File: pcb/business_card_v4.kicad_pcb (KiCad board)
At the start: 16 copper layers, 89 x 51 mm, 69 parts, among them J1 Conn_01x05_Male, J2 Conn_01x01_Male, SW1 SW_SPST, U1 MIC5504-3.3YM5, U2 STM32G030F6P6

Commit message: create a net and update version of file names
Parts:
- removed JP1: USBPCB, business_card_v1:USB-A-PCB
- added J3: USB_A, Kevin-Lutzer-Kicad-Lbr:USB-A-PCB, F.Cu at (112.0, 122.5)
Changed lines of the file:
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@@
     (add_net SWDIO)
+  )
+  (module Kevin-Lutzer-Kicad-Lbr:USB-A-PCB (layer Top)
+    (at 111.96828 122.5423 45)
+    (descr "Card-edge USB A connector.\n\nFor boards designed to be plugged directly into a USB slot. If possible, ensure that your PCB is about 2.4mm thick to fit snugly.")
+    (fp_text reference J3 (at 0 -7.1 45) (layer F.SilkS) hide
+      (effects (font (size 1.27 1.27) (thickness 0.15)))
+    )
+    (fp_text value USB_A (at 0 7.5 45) (layer F.SilkS) hide
+      (effects (font (size 1.27 1.27) (thickness 0.15)))
+    )
+    (fp_line (start -5 6) (end -5 -6) (layer F.Fab) (width 0.127))
+    (fp_line (start 3.7 6) (end -5 6) (layer F.Fab) (width 0.127))
+    (fp_line (start 3.7 -6) (end 3.7 6) (layer F.Fab) (width 0.127))
+    (fp_line (start -5 -6) (end 3.7 -6) (layer F.Fab) (width 0.127))
+    (pad 4 smd rect (at -0.2 -3.5 45) (size 7.5 1.5) (layers Top F.Paste F.Mask)
+      (net 1 GND) (solder_mask_margin 0.1016))
+    (pad 3 smd rect (at 0.3 -1 45) (size 6.5 1) (layers Top F.Paste F.Mask)
+      (solder_mask_margin 0.1016))
+    (pad 2 smd rect (at 0.3 1 45) (size 6.5 1) (layers Top F.Paste F.Mask)
+      (solder_mask_margin 0.1016))
+    (pad 1 smd rect (at -0.2 3.5 45) (size 7.5 1.5) (layers Top F.Paste F.Mask)
+      (net 2 +5V) (solder_mask_margin 0.1016))
   )
   (module Resistor_SMD:R_0805_2012Metric (layer Top)
@@
     )
   )
-  (module business_card_v1:USB-A-PCB (layer Top)
-    (at 111.96828 122.5423 45)
-    (descr "Card-edge USB A connector.\n\nFor boards designed to be plugged directly into a USB slot. If possible, ensure that your PCB is about 2.4mm thick to fit snugly.")
-    (fp_text reference JP1 (at 0 0 45) (layer F.SilkS) hide
-      (effects (font (size 1.27 1.27) (thickness 0.15)))
-    )
-    (fp_text value USBPCB (at -1.270002 5.079999 45) (layer F.SilkS) hide
-      (effects (font (size 0.38608 0.38608) (thickness 0.030886)))
-    )
-    (fp_text user "Card edge" (at -6.392146 -3.543609 135) (layer Cmts.User) hide
-      (effects (font (size 0.9652 0.9652) (thickness 0.08128)) (justify left bottom))
-    )
-    (fp_text user >Value (at -1.27 5.08 45) (layer F.Fab) hide
-      (effects (font (size 0.38608 0.38608) (thickness 0.032512)) (justify left bottom))
-    )
-    (fp_text user >Name (at -1.27 -5.08 45) (layer F.SilkS) hide
-      (effects (font (size 0.38608 0.38608) (thickness 0.032512)) (justify left bottom))
-    )
-    (fp_line (start -5 6) (end -5 -6) (layer F.Fab) (width 0.127))
-    (fp_line (start 3.7 6) (end -5 6) (layer F.Fab) (width 0.127))
-    (fp_line (start 3.7 -6) (end 3.7 6) (layer F.Fab) (width 0.127))
-    (fp_line (start -5 -6) (end 3.7 -6) (layer F.Fab) (width 0.127))
-    (pad GND smd rect (at -0.2 -3.5 45) (size 7.5 1.5) (layers Top F.Paste F.Mask)
-      (net 1 GND) (solder_mask_margin 0.1016))
-    (pad USB_P smd rect (at 0.3 -1 45) (size 6.5 1) (layers Top F.Paste F.Mask)
-      (solder_mask_margin 0.1016))
-    (pad USB_M smd rect (at 0.3 1 45) (size 6.5 1) (layers Top F.Paste F.Mask)
-      (solder_mask_margin 0.1016))
-    (pad 5V smd rect (at -0.2 3.5 45) (size 7.5 1.5) (layers Top F.Paste F.Mask)
-      (net 2 +5V) (solder_mask_margin 0.1016))
-  )
   (module Button_Switch_SMD:SW_Push_1P1T_NO_CK_KMR2 (layer Top)
     (at 146.2 121.5)
@@
     (effects (font (size 1 1) (thickness 0.14224)))
   )
-  (gr_text 5v-SUP (at 122 110.85) (layer B.SilkS)
+  (gr_text 5v-SUP (at 121.9 110.85) (layer B.SilkS)
     (effects (font (size 1 1) (thickness 0.14224)) (justify mirror))
   )

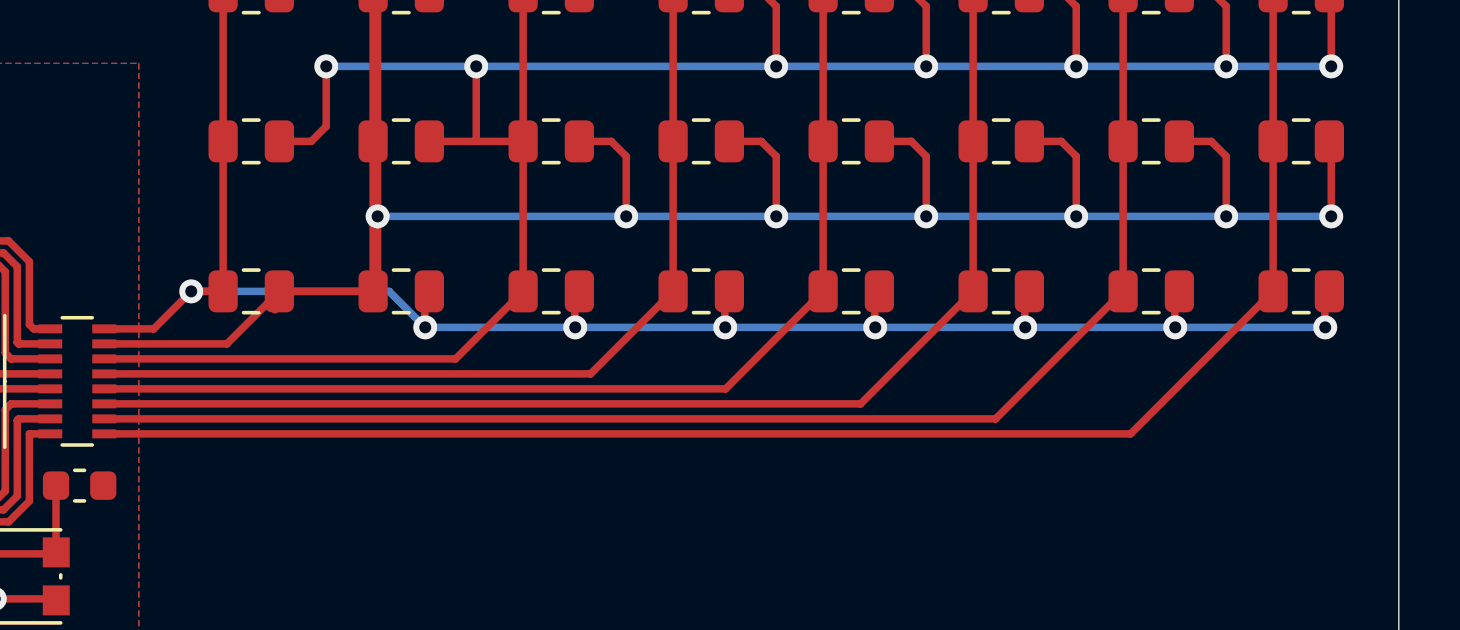
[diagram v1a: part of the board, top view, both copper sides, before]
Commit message: update pcb gerbers
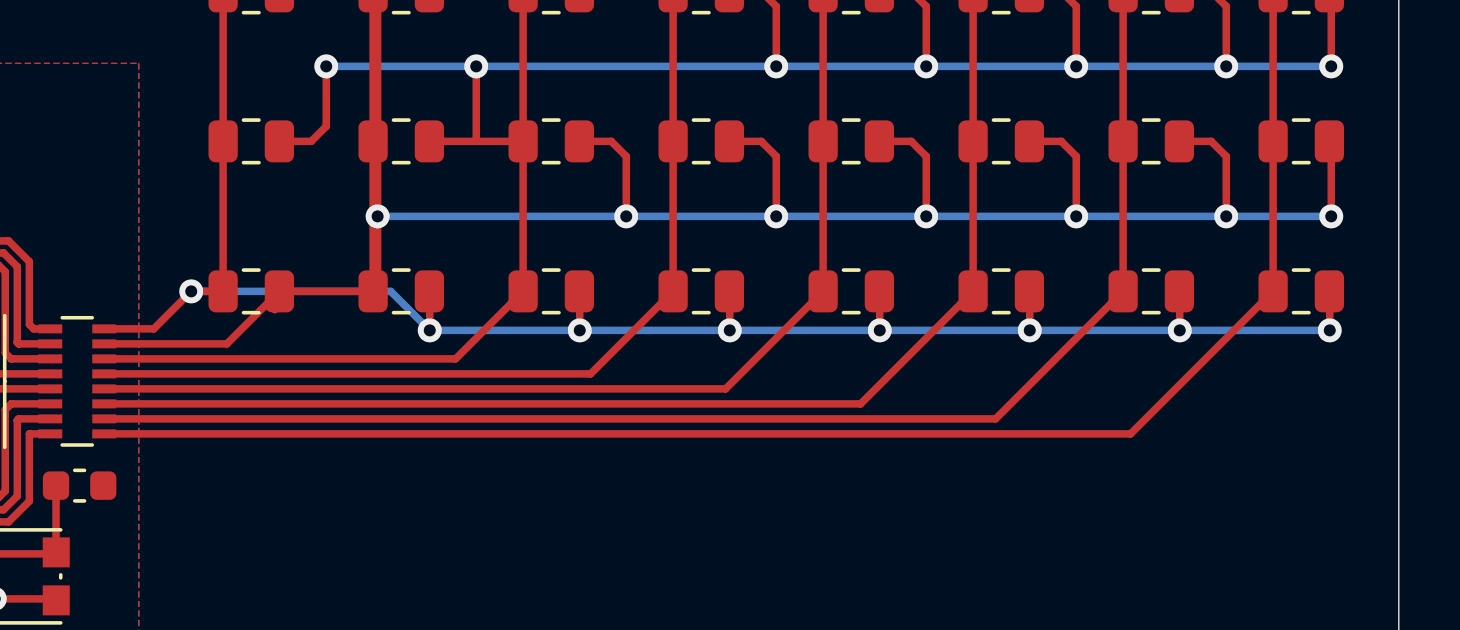
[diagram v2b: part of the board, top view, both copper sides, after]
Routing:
- net Net-(D1-Pad2): track 82.4 -> 83.2 mm
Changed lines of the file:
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@@
   (gr_line (start 104.0127 130.497741) (end 104.01265 130.49716) (layer Dwgs.User) (width 0.025))
   (gr_line (start 104.01265 130.49716) (end 104.012509 130.496419) (layer Dwgs.User) (width 0.025))
+  (via (at 160.7 113.3) (size 0.8) (drill 0.4) (layers Top Bottom) (net 15))
   (segment (start 109.334205 120.221548) (end 109.334205 120.218295) (width 0.25) (layer Top) (net 1) (status 30))
   (segment (start 109.334205 120.218295) (end 109.397705 120.218295) (width 0.25) (layer Top) (net 1) (status 30))
@@
   (segment (start 140.8725 112.138) (end 140.8725 112.759242) (width 0.25) (layer Top) (net 14) (status 30))
   (segment (start 140.8725 110) (end 140.8725 112.138) (width 0.25) (layer Top) (net 14) (status 30))
-  (via (at 190.55 113.2) (size 0.8) (drill 0.4) (layers Top Bottom) (net 15))
   (segment (start 153.9625 112) (end 153.9625 111.525) (width 0.25) (layer Top) (net 15) (status 30))
-  (segment (start 190.5375 113.1875) (end 190.55 113.2) (width 0.25) (layer Top) (net 15))
-  (segment (start 190.5375 112) (end 190.5375 113.1875) (width 0.25) (layer Top) (net 15) (status 10))
-  (via (at 185.55 113.2) (size 0.8) (drill 0.4) (layers Top Bottom) (net 15))
-  (via (at 180.55 113.2) (size 0.8) (drill 0.4) (layers Top Bottom) (net 15))
-  (via (at 175.55 113.2) (size 0.8) (drill 0.4) (layers Top Bottom) (net 15))
-  (via (at 170.55 113.2) (size 0.8) (drill 0.4) (layers Top Bottom) (net 15))
-  (via (at 165.55 113.2) (size 0.8) (drill 0.4) (layers Top Bottom) (net 15))
-  (via (at 160.55 113.2) (size 0.8) (drill 0.4) (layers Top Bottom) (net 15))
-  (segment (start 160.55 113.2) (end 190.55 113.2) (width 0.25) (layer Bottom) (net 15))
-  (segment (start 185.5375 113.1875) (end 185.55 113.2) (width 0.25) (layer Top) (net 15))
-  (segment (start 185.5375 112) (end 185.5375 113.1875) (width 0.25) (layer Top) (net 15) (status 10))
-  (segment (start 180.5375 113.1875) (end 180.55 113.2) (width 0.25) (layer Top) (net 15))
-  (segment (start 180.5375 112) (end 180.5375 113.1875) (width 0.25) (layer Top) (net 15) (status 10))
-  (segment (start 175.5375 113.1875) (end 175.55 113.2) (width 0.25) (layer Top) (net 15))
-  (segment (start 175.5375 112) (end 175.5375 113.1875) (width 0.25) (layer Top) (net 15) (status 10))
-  (segment (start 160.5375 113.1875) (end 160.55 113.2) (width 0.25) (layer Top) (net 15))
-  (segment (start 160.5375 112) (end 160.5375 113.1875) (width 0.25) (layer Top) (net 15) (status 10))
-  (segment (start 165.5375 113.1875) (end 165.55 113.2) (width 0.25) (layer Top) (net 15))
-  (segment (start 165.5375 112) (end 165.5375 113.1875) (width 0.25) (layer Top) (net 15) (status 10))
-  (segment (start 170.5375 113.1875) (end 170.55 113.2) (width 0.25) (layer Top) (net 15))
-  (segment (start 170.5375 112) (end 170.5375 113.1875) (width 0.25) (layer Top) (net 15) (status 10))
   (segment (start 153.95 112.0125) (end 153.9625 112) (width 0.25) (layer Top) (net 15) (status 30))
   (segment (start 153.8125 82) (end 153.8125 112) (width 0.25) (layer Top) (net 15) (status 30))
-  (segment (start 152.5 112) (end 159.35 112) (width 0.25) (layer Bottom) (net 15))
-  (segment (start 159.35 112) (end 160.55 113.2) (width 0.25) (layer Bottom) (net 15))
   (segment (start 152.5 112) (end 153.9625 112) (width 0.25) (layer Top) (net 15) (status 20))
   (via (at 152.75 112) (size 0.8) (drill 0.4) (layers Top Bottom) (net 15))
   (segment (start 151.5 113.25) (end 152.75 112) (width 0.25) (layer Top) (net 15))
   (segment (start 149.85 113.25) (end 151.5 113.25) (width 0.25) (layer Top) (net 15) (status 10))
+  (via (at 165.7 113.3) (size 0.8) (drill 0.4) (layers Top Bottom) (net 15))
+  (via (at 170.7 113.3) (size 0.8) (drill 0.4) (layers Top Bottom) (net 15))
+  (via (at 175.7 113.3) (size 0.8) (drill 0.4) (layers Top Bottom) (net 15))
+  (via (at 180.7 113.3) (size 0.8) (drill 0.4) (layers Top Bottom) (net 15))
+  (via (at 185.7 113.3) (size 0.8) (drill 0.4) (layers Top Bottom) (net 15))
+  (via (at 190.7 113.3) (size 0.8) (drill 0.4) (layers Top Bottom) (net 15))
+  (segment (start 160.7 112.0125) (end 160.6875 112) (width 0.25) (layer Top) (net 15))
+  (segment (start 160.7 113.3) (end 160.7 112.0125) (width 0.25) (layer Top) (net 15))
+  (segment (start 165.7 112.0125) (end 165.6875 112) (width 0.25) (layer Top) (net 15))
+  (segment (start 165.7 113.3) (end 165.7 112.0125) (width 0.25) (layer Top) (net 15))
+  (segment (start 170.7 112.0125) (end 170.6875 112) (width 0.25) (layer Top) (net 15))
+  (segment (start 170.7 113.3) (end 170.7 112.0125) (width 0.25) (layer Top) (net 15))
+  (segment (start 175.7 112.0125) (end 175.6875 112) (width 0.25) (layer Top) (net 15))
+  (segment (start 175.7 113.3) (end 175.7 112.0125) (width 0.25) (layer Top) (net 15))
+  (segment (start 180.7 112.0125) (end 180.6875 112) (width 0.25) (layer Top) (net 15))
+  (segment (start 180.7 113.3) (end 180.7 112.0125) (width 0.25) (layer Top) (net 15))
+  (segment (start 185.7 112.0125) (end 185.6875 112) (width 0.25) (layer Top) (net 15))
+  (segment (start 185.7 113.3) (end 185.7 112.0125) (width 0.25) (layer Top) (net 15))
+  (segment (start 190.7 112.0125) (end 190.6875 112) (width 0.25) (layer Top) (net 15))
+  (segment (start 190.7 113.3) (end 190.7 112.0125) (width 0.25) (layer Top) (net 15))
+  (segment (start 159.4 112) (end 160.7 113.3) (width 0.25) (layer Bottom) (net 15))
+  (segment (start 152.5 112) (end 159.4 112) (width 0.25) (layer Bottom) (net 15))
+  (segment (start 160.7 113.3) (end 190.7 113.3) (width 0.25) (layer Bottom) (net 15))
   (segment (start 188.8125 82) (end 188.8125 112) (width 0.25) (layer Top) (net 16) (status 30))
   (segment (start 187.83509 81.02259) (end 188.8125 82) (width 0.25) (layer Top) (net 16) (status 20))
